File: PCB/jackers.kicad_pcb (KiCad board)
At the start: 2 copper layers, 95.1 x 98.5 mm, 12 parts, among them SW1 SW_Push, SW2 SW_Push, SW3 SW_Push, SW4 SW_Push, SW5 SW_Push, SW6 SW_Push, SW7 SW_Push, SW8 SW_Push, SW9 SW_Push, U1 XIAO-RP2040-DIP

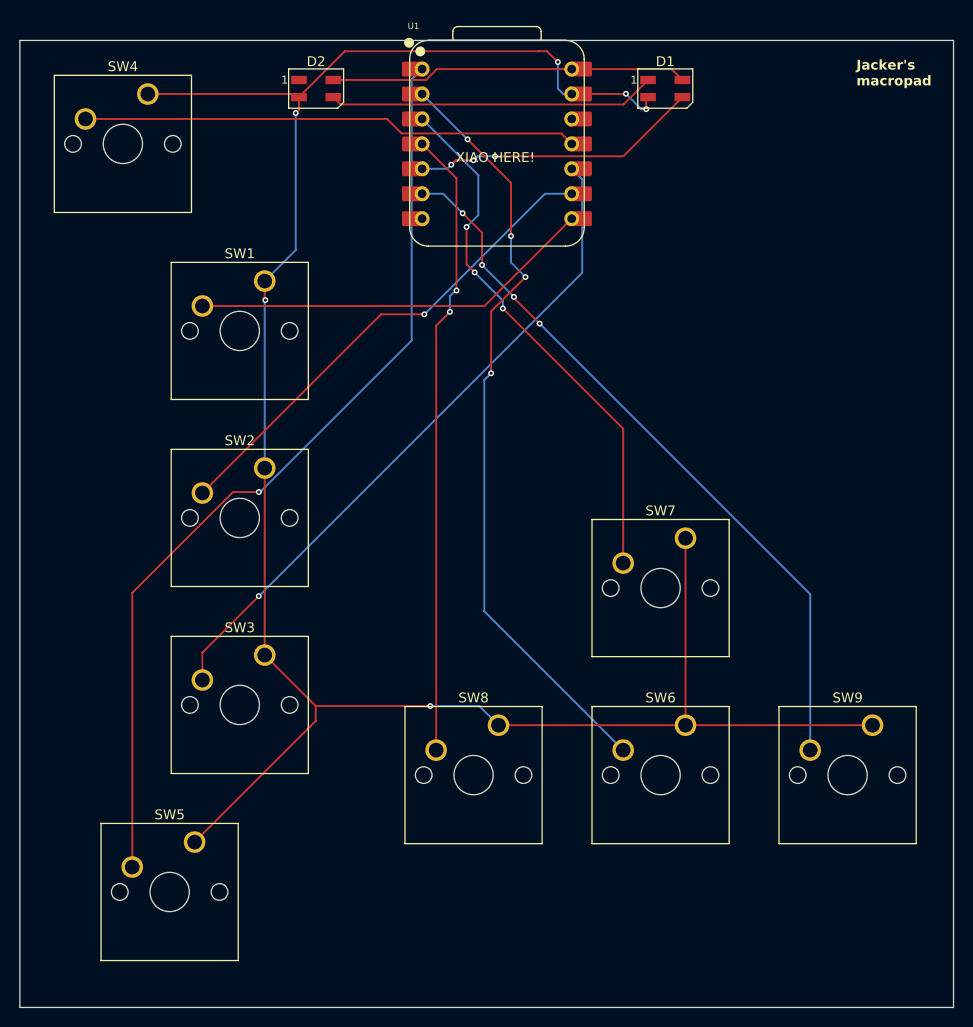
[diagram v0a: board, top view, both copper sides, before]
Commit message: Updated PCB
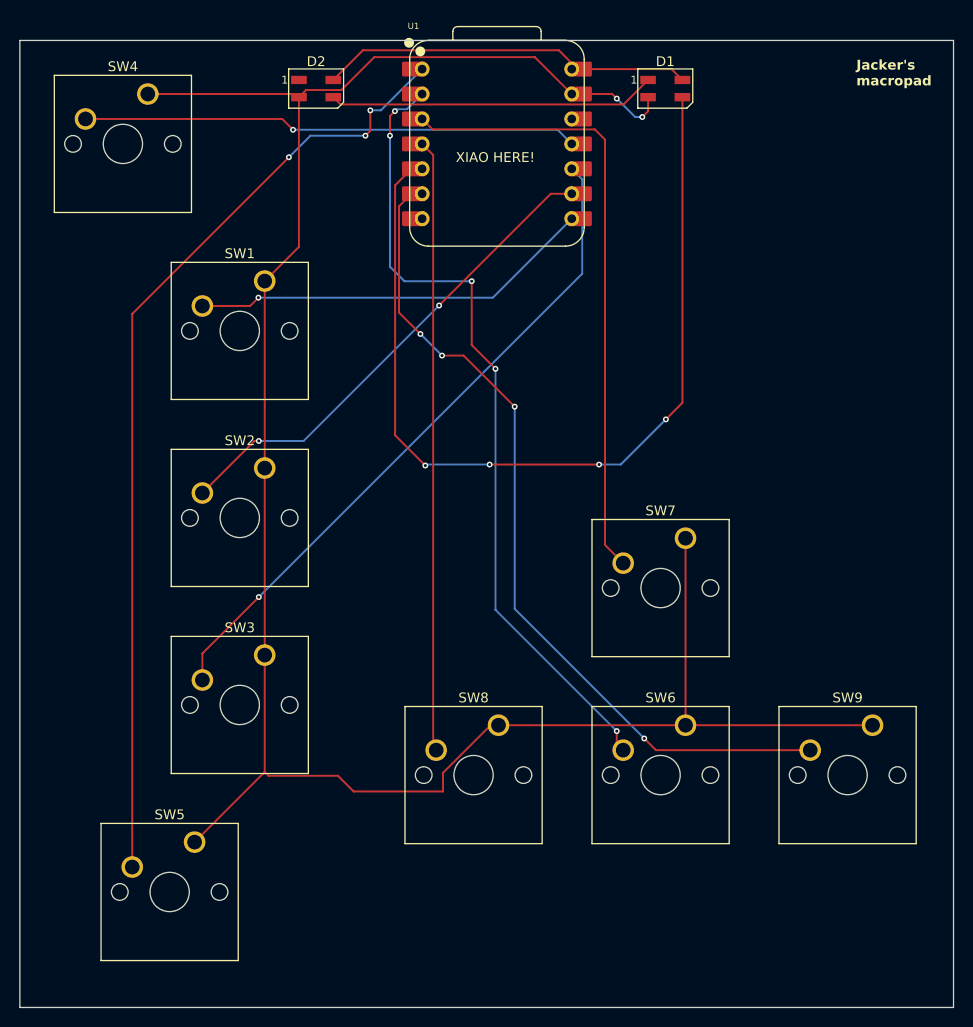
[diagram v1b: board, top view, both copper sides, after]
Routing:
- net Net-(D1-DIN): track 29.5 -> 93.6 mm, vias 3 -> 4
- net Net-(U1-GPIO7/SCL): track 74.6 -> 86.1 mm
- net Net-(U1-GPIO28/ADC2/A2): track 54.7 -> 63.4 mm, vias 3 -> 0
- net Net-(U1-GPIO27/ADC1/A1): track 78.8 -> 82.6 mm, vias 4 -> 5
- net GND: track 218.6 -> 222.1 mm, vias 6 -> 2
- net Net-(U1-GPIO26/ADC0/A0): track 95.1 -> 97.4 mm, vias 1 -> 3
- net +5V: track 35.6 -> 37.6 mm
- net Net-(U1-GPIO29/ADC3/A3): track 64.1 -> 62.3 mm, vias 2 -> 0
- net Net-(U1-GPIO3/MOSI): vias 0 -> 1
- net Net-(U1-GPIO2/SCK): vias 1 -> 2
- net Net-(U1-GPIO1/RX): vias 0 -> 1
